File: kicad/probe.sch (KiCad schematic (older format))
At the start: 11 parts

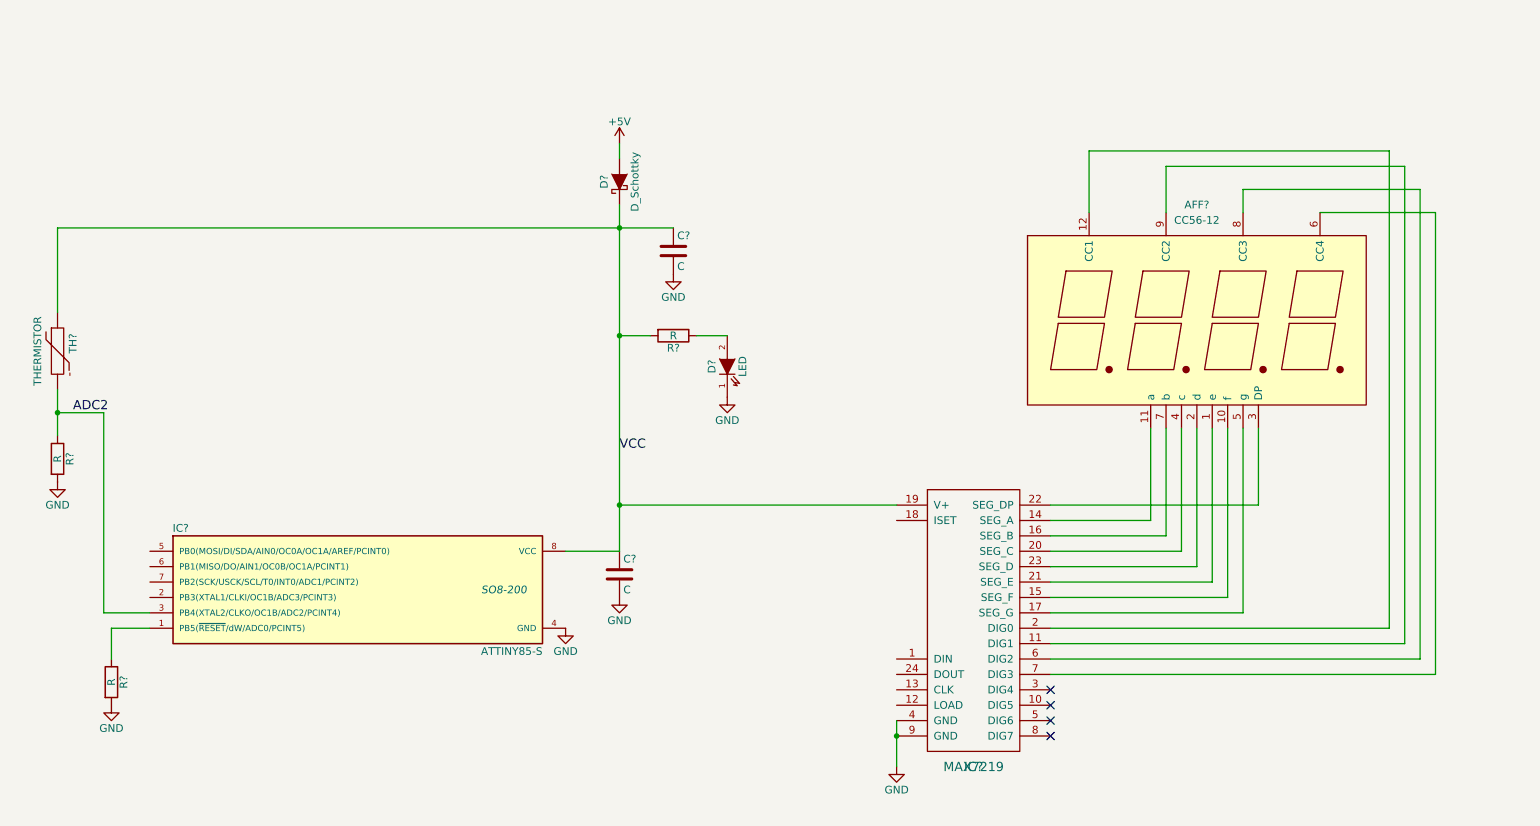
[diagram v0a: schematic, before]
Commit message: Schematic v0.1
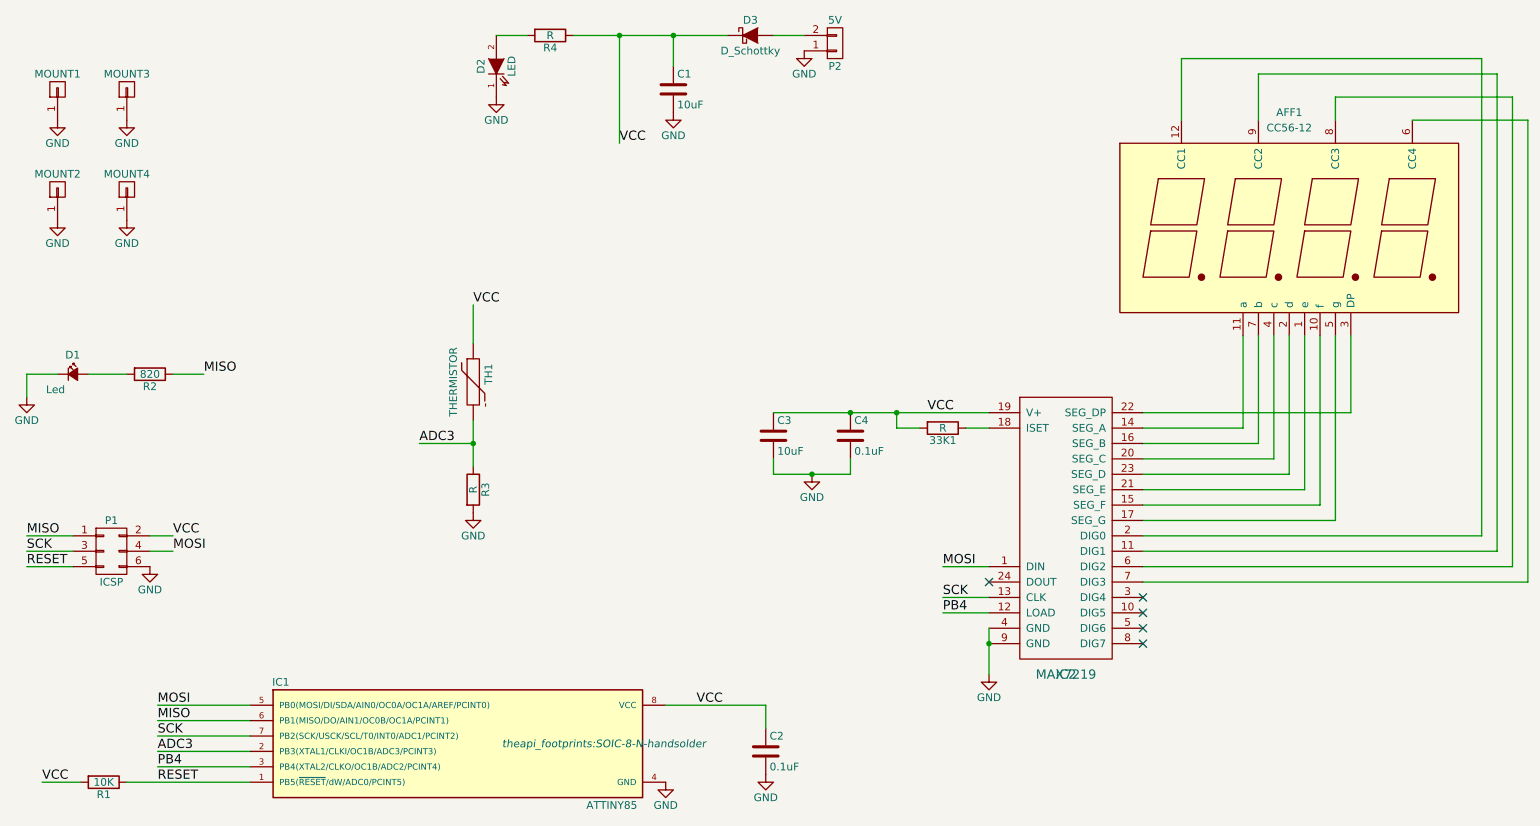
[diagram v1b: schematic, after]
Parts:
- removed C? (x2): C, symbol C
- removed D?: D_Schottky, symbol D_Schottky
- removed IC?: ATTINY85-S, SO8-200, symbol ATTINY85-S
- removed R?: R, symbol R
- added 33K1: R, Resistors_SMD:R_0805_HandSoldering, symbol R
- added C1, C3: 10uF, Capacitors_SMD:C_0805_HandSoldering, symbol C
- added C2, C4: 0.1uF, Capacitors_SMD:C_0805_HandSoldering, symbol C
- added D1: Led, theapi_footprints:LED_0805, symbol Led_Small
- added D3: D_Schottky, theapi_footprints:SOD-123-Schottky, symbol D_Schottky
- added IC1: ATTINY85, theapi_footprints:SOIC-8-N-handsolder, symbol ATTINY85-S
- added MOUNT1, MOUNT2, MOUNT3, MOUNT4: CONN_01X01, Pin_Headers:Pin_Header_Straight_1x01, symbol CONN_01X01
- added P1: ICSP, Pin_Headers:Pin_Header_Straight_2x03, symbol CONN_02X03
- added P2: 5V, Pin_Headers:Pin_Header_Straight_1x02, symbol CONN_01X02
- added R1: 10K, Resistors_SMD:R_0805_HandSoldering, symbol R
- added R2: 820, Resistors_SMD:R_0805_HandSoldering, symbol R
- AFF1: renamed from AFF?; footprint (none) -> Displays_7-Segment:Cx56-12
- D2: renamed from D?; footprint (none) -> theapi_footprints:LED_0805
- IC2: renamed from IC?; footprint (none) -> Housings_DIP:DIP-24_W15.24mm
- R3, R4: renamed from R?; footprint (none) -> Resistors_SMD:R_0805_HandSoldering
- TH1: renamed from TH?; footprint (none) -> Discret:R1
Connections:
- net GND: now also C1.2, C2.2, C3.2, C4.2, D1.1 (K), IC1.4 (GND), MOUNT1.1 (P1), MOUNT2.1 (P1), MOUNT3.1 (P1), MOUNT4.1 (P1), P1.6 (P6), P2.1 (P1)
- net VCC: now also R4.1, 33K1.2, C1.1, C2.1, C3.1, C4.1, D3.1 (K), IC1.8 (VCC), P1.2 (P2), R1.2; no longer R4.2
- net at D2.2 (A): now also R4.2; no longer R4.1
- net MOSI: now reaches IC2.1 (DIN)
- net MOSI: now also IC1.5 (PB0(MOSI/DI/SDA/AIN0/OC0A/OC1A/AREF/PCINT0)), P1.4 (P4)
- net PB4: now reaches IC2.12 (LOAD)
- net PB4: now also IC1.3 (PB4(XTAL2/CLKO/OC1B/ADC2/PCINT4))
- net SCK: now reaches IC2.13 (CLK)
- net SCK: now also IC1.7 (PB2(SCK/USCK/SCL/T0/INT0/ADC1/PCINT2)), P1.3 (P3)
- net at IC2.18 (ISET): now also 33K1.1
- net ADC2 renamed ADC3
- net ADC3: now also IC1.2 (PB3(XTAL1/CLKI/OC1B/ADC3/PCINT3))
- new net: D1.2 (A), R2.2
- new net: D3.2 (A), P2.2 (P2)
- new net MISO: IC1.6 (PB1(MISO/DO/AIN1/OC0B/OC1A/PCINT1)), P1.1 (P1), R2.1
- new net RESET: IC1.1 (PB5(~RESET~/dW/ADC0/PCINT5)), P1.5 (P5), R1.1
- no-connect marks 4 -> 5
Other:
- moved on the sheet: AFF1, D2, IC2, R3, R4, TH1

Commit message: Initial layout
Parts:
- IC2: footprint Housings_DIP:DIP-24_W15.24mm -> Housings_DIP:DIP-24_W7.62mm_LongPads
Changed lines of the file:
@@
 F 0 "IC2" H 7900 5200 60  0000 C CNN
 F 1 "MAX7219" H 7900 5200 60  0000 C CNN
-F 2 "Housings_DIP:DIP-24_W15.24mm" H 7900 5200 60  0001 C CNN
+F 2 "Housings_DIP:DIP-24_W7.62mm_LongPads" H 7900 5200 60  0001 C CNN
 F 3 "" H 7900 5200 60  0000 C CNN
 	1    7900 5200
